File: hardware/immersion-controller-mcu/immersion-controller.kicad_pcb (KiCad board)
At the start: 2 copper layers, 144.8 x 45.7 mm, 14 parts, among them J1 TANK-TOP, J2 TANK-BOTTOM, J3 COLD, J4 DISPLAY, J5 RTC, J7 MCU, SW2 RotaryEncoder_Switch, U1 ESP32-S3-DevKitC, U12 DHT11

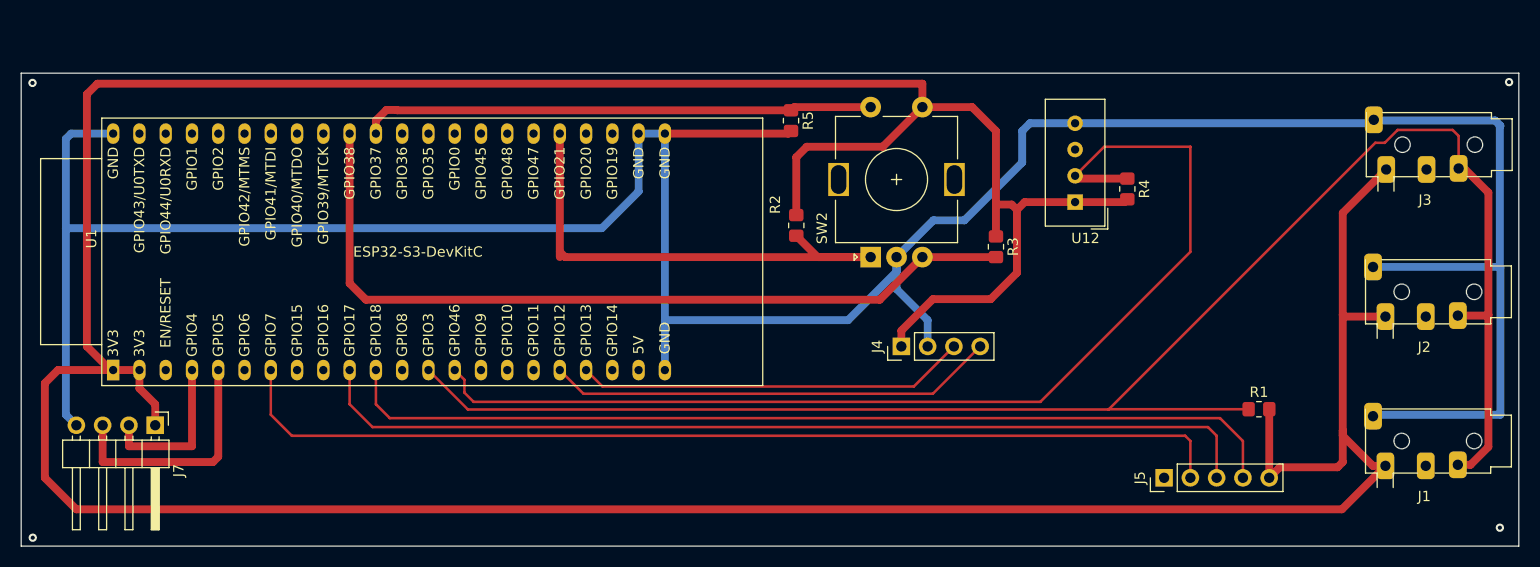
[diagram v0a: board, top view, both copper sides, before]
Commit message: Initial Prototype results
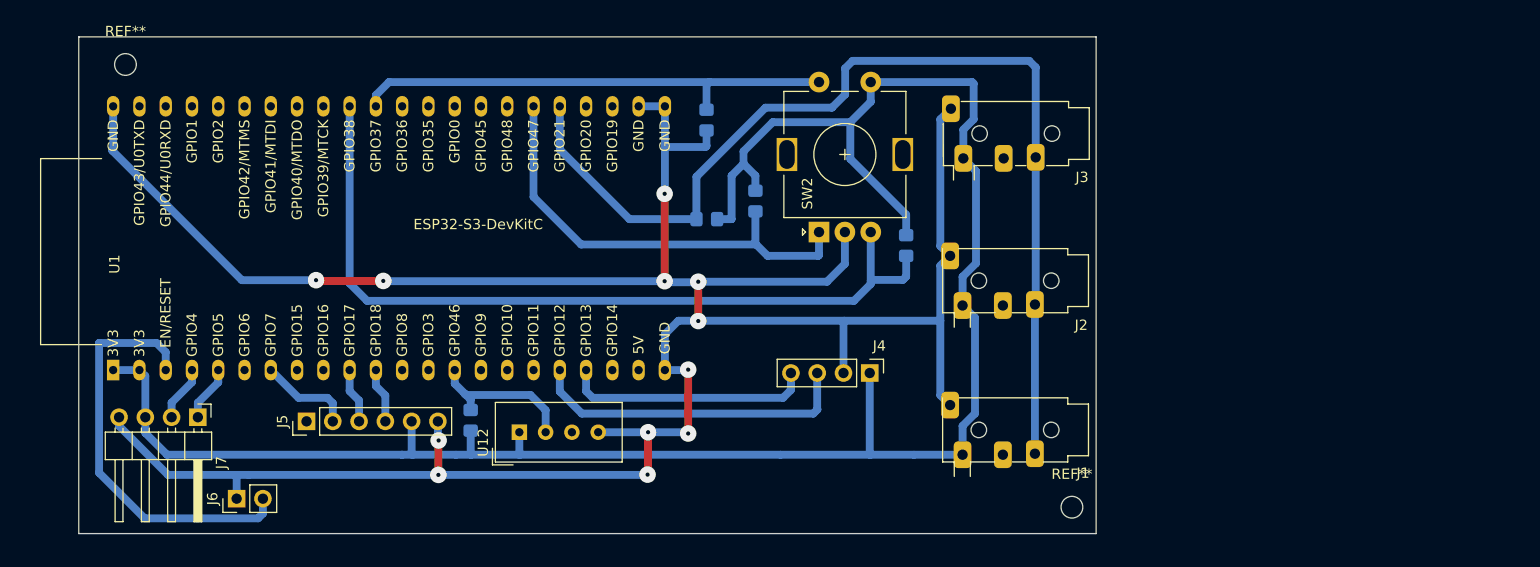
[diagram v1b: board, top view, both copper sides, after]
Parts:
- added J6: Conn_01x02_Pin, Connector_PinHeader_2.54mm:PinHeader_1x02_P2.54mm_Vertical, F.Cu at (33.3, 119.9)
- added REF**: MountingHole_2.1mm, MountingHole:MountingHole_2.1mm, F.Cu at (22.5, 77.9)
- added REF**: MountingHole_2.1mm, MountingHole:MountingHole_2.1mm, F.Cu at (114.0, 120.7)
- J5: footprint Connector_PinHeader_2.54mm:PinHeader_1x05_P2.54mm_Vertical -> Connector_PinHeader_2.54mm:PinHeader_1x06_P2.54mm_Vertical
- R1, R2, R3, R4, R5: moved to B.Cu
- moved J5 83.1 mm to (40.0, 112.4)
- moved R4 67.3 mm to (55.9, 112.3)
- moved U12 58.2 mm to (60.6, 113.5), turned to 90 degrees
- moved R1 56.5 mm to (78.7, 92.8)
- moved J1 40.9 mm to (107.2, 113.2)
- moved J2 40.9 mm to (107.2, 98.8)
- moved J3 40.9 mm to (107.3, 84.6)
- moved R3 8.68 mm to (98.0, 95.4)
- moved R5 8.17 mm to (78.7, 83.3)
- moved SW2 5.55 mm to (89.6, 94.1)
- moved R2 4.60 mm to (83.4, 91.1)
- moved J7 4.20 mm to (29.5, 112.0)
- moved J4 3.99 mm to (94.5, 107.7), turned to -90 degrees
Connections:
- J7 pad 1: +3.3V -> RELAY_BOTTOM
- J7 pad 3: RELAY_BOTTOM -> +3.3V
- U1 pad 13: WATERTEMP_DATA -> unconnected-(U1-GPIO3/ADC1_CH2-Pad13)
- U1 pad 18: DISPLAY_SDA -> DISPLAY_SCL
- U1 pad 19: DISPLAY_SCL -> DISPLAY_SDA
- U1 pad 27: ROT_CLK -> WATERTEMP_DATA
- U1 pad 28: unconnected-(U1-GPIO47-Pad28) -> ROT_CLK
- U1 pad 3: unconnected-(U1-CHIP_PU-Pad3) -> RESET
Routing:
- net +3.3V: track 395.5 -> 194.0 mm
- net DHT_DATA: track 106.8 -> 15.1 mm
- net RTC_SQW: track 97.8 -> 9.08 mm
- net RTC_SCK: track 92.4 -> 5.34 mm
- net RTC_SDA: track 92.2 -> 5.34 mm
- net WATERTEMP_DATA: track 164.4 -> 100.8 mm
- net RESET: track 0.00 -> 40.4 mm
- net GND: track 287.2 -> 261.3 mm, vias 0 -> 12
- net DISPLAY_SDA: track 43.5 -> 24.1 mm
- net RELAY_BOTTOM: track 23.3 -> 5.37 mm
- net RELAY_TOP: track 15.5 -> 5.37 mm
- net DISPLAY_SCL: track 37.8 -> 31.6 mm
- net ROT_CLK: track 50.2 -> 44.2 mm
- net ROT_SW: track 49.7 -> 47.7 mm
- net (no net): vias 4 -> 0
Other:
- board size 144.8 x 45.7 mm -> 98.4 x 48 mm
